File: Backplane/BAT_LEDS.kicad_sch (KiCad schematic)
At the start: 15 parts, among them U10 SN74LVC1G125DBVR, U11 SN74LVC1G125DBVR, U14 SN74LVC1G125DBVR, U17 SN74LVC1G125DBVR, U18 SN74LVC1G125DBVR

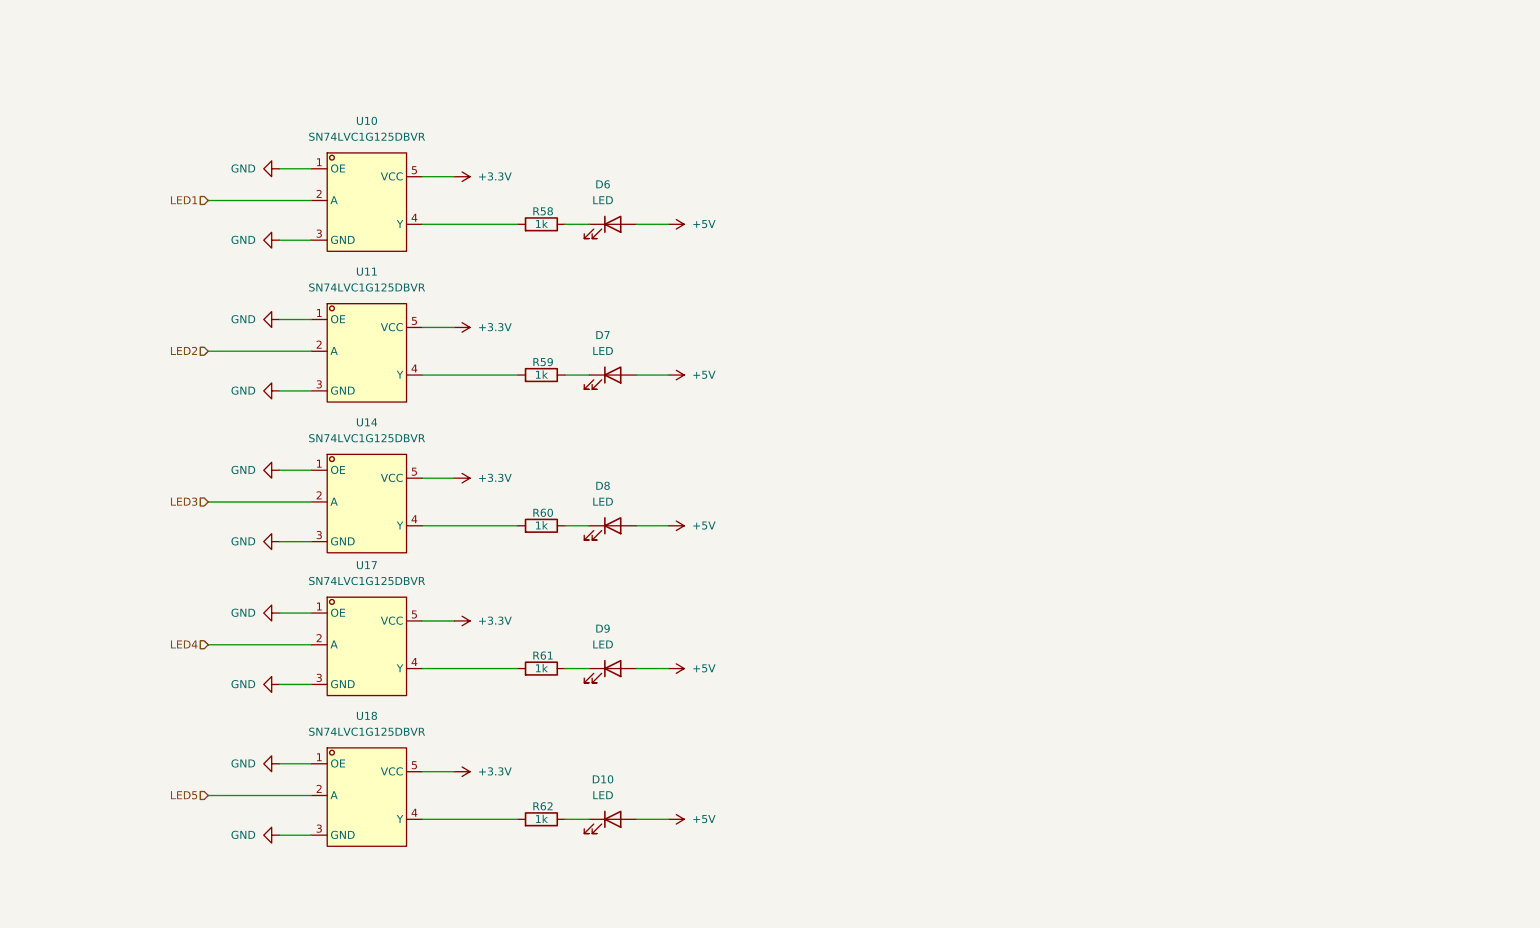
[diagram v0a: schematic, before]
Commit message: Starting to work on layout.
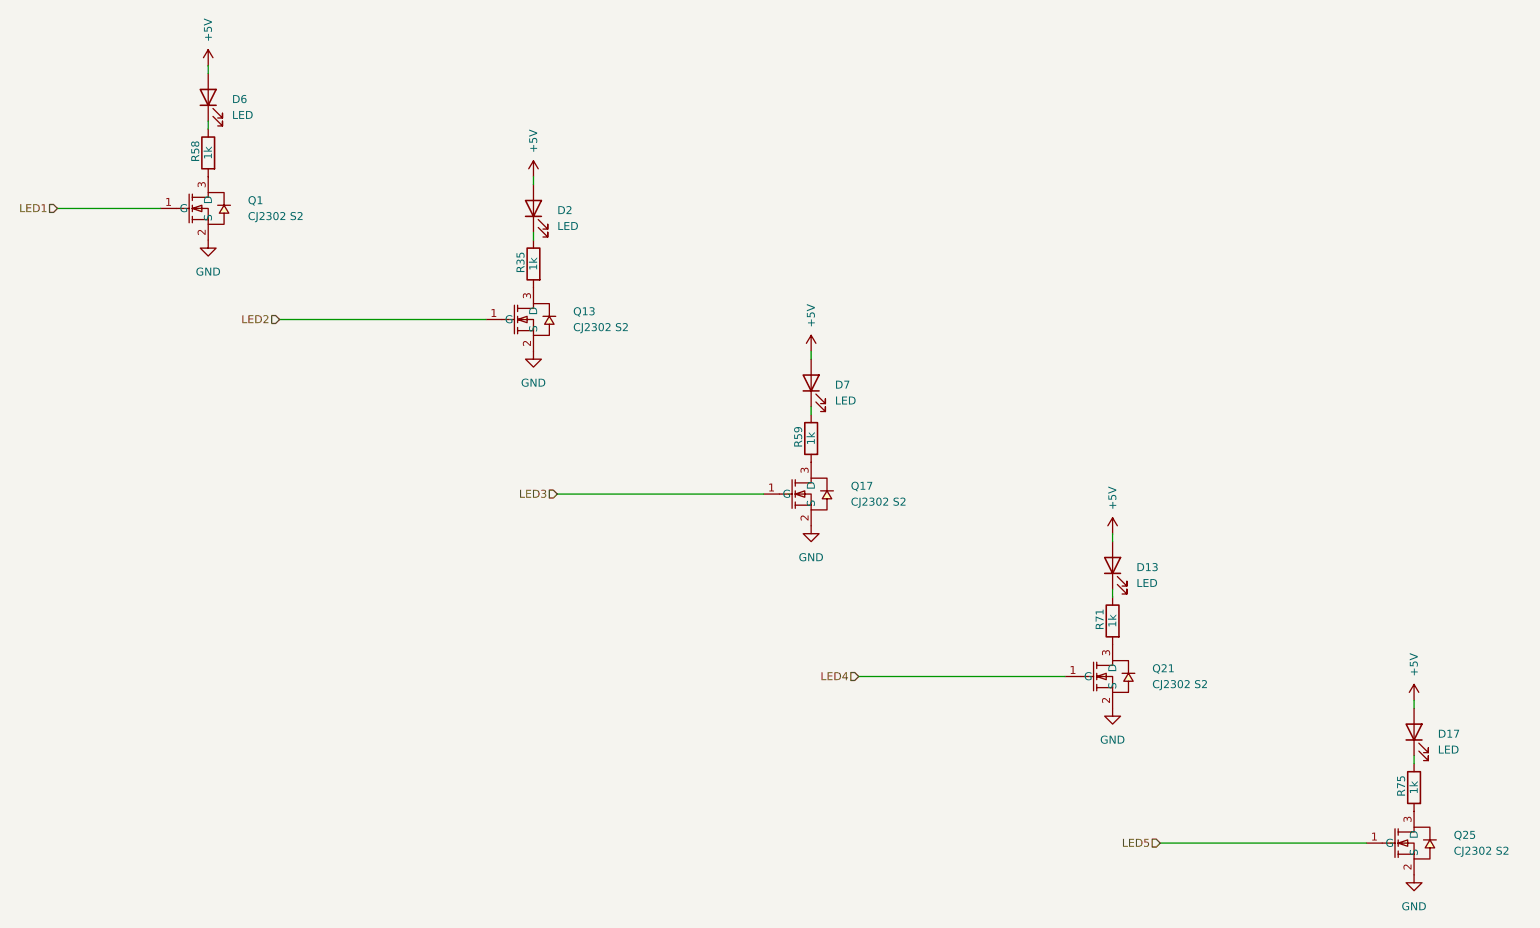
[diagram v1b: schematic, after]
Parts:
- removed D10, D8, D9: LED, symbol Device:LED
- removed R60, R61, R62: 1k, Resistor_SMD:R_1206_3216Metric_Pad1.30x1.75mm_HandSolder, symbol Device:R
- removed U10, U11, U14, U17, U18: SN74LVC1G125DBVR, COMPONENTS:SOT-23-5_L3.0-W1.7-P0.95-LS2.8-BL, symbol COMPONENTS:SN74LVC1G125DBVR
- added D13, D17, D2: LED, LED_SMD:LED_1206_3216Metric, symbol Device:LED
- added Q1, Q13, Q17, Q21, Q25: CJ2302 S2, COMPONENTS:SOT-23-3_L3.0-W1.7-P0.95-LS2.9-BR, symbol COMPONENTS:CJ2302S2
- added R35, R71, R75: 1k, Resistor_SMD:R_1206_3216Metric_Pad1.30x1.75mm_HandSolder, symbol Device:R
- D6, D7: footprint (none) -> LED_SMD:LED_1206_3216Metric
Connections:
- net +5V: now also D13.2 (A), D17.2 (A), D2.2 (A)
- net GND: now also Q1.2 (S), Q13.2 (S), Q17.2 (S), Q21.2 (S), Q25.2 (S)
- net LED1: now also Q1.1 (G)
- net LED2: now also Q13.1 (G)
- net LED3: now also Q17.1 (G)
- net LED4: now also Q21.1 (G)
- net LED5: now also Q25.1 (G)
- net at R59.2: now also Q17.3 (D)
- net at R58.2: now also Q1.3 (D)
- new net: Q13.3 (D), R35.2
- new net: D13.1 (K), R71.1
- new net: Q21.3 (D), R71.2
- new net: Q25.3 (D), R75.2
- new net: D17.1 (K), R75.1
- new net: D2.1 (K), R35.1
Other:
- moved on the sheet: D6, R58
